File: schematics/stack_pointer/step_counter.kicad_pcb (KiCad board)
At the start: 2 copper layers, 100 x 91 mm, 17 parts, among them U1 74HC00, U2 74HC193, U3 74HC193, U4 74HC193, U5 74HC193, U6 74HC245, U7 74HC245

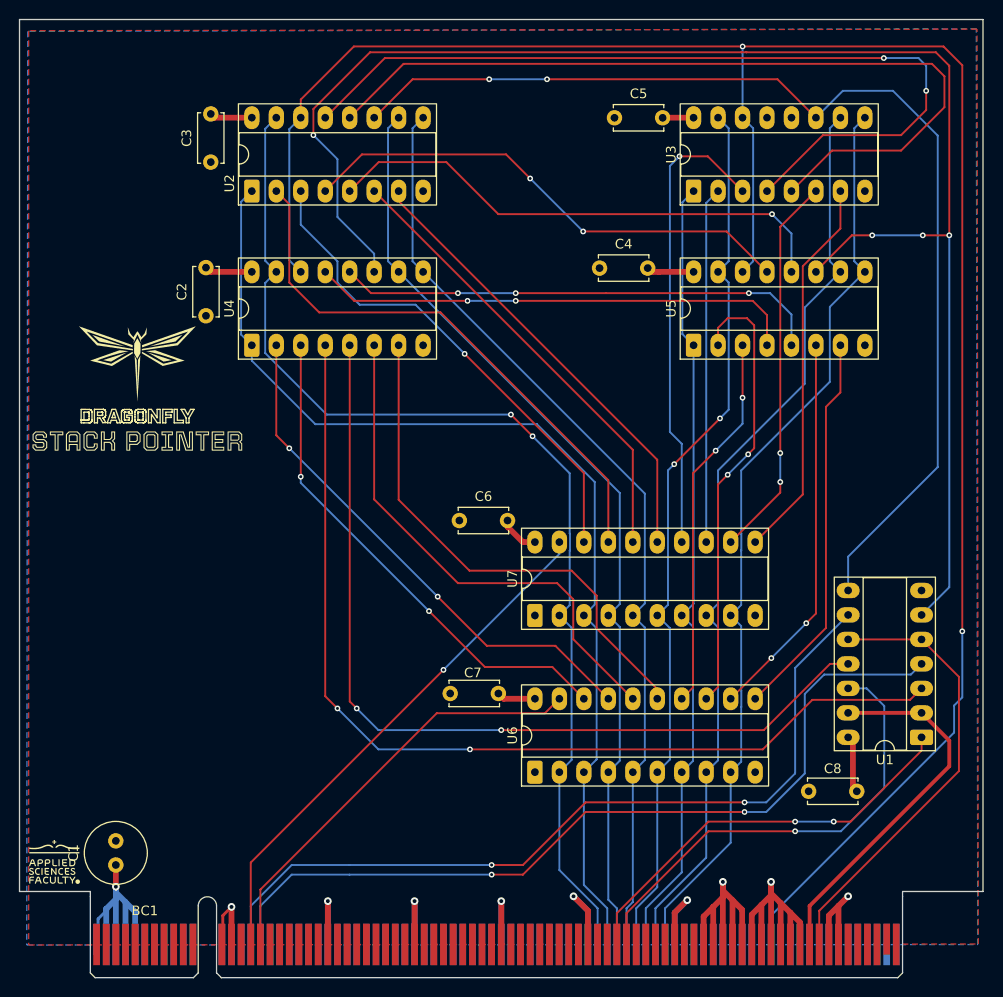
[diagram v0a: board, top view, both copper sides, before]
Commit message: silklayer check
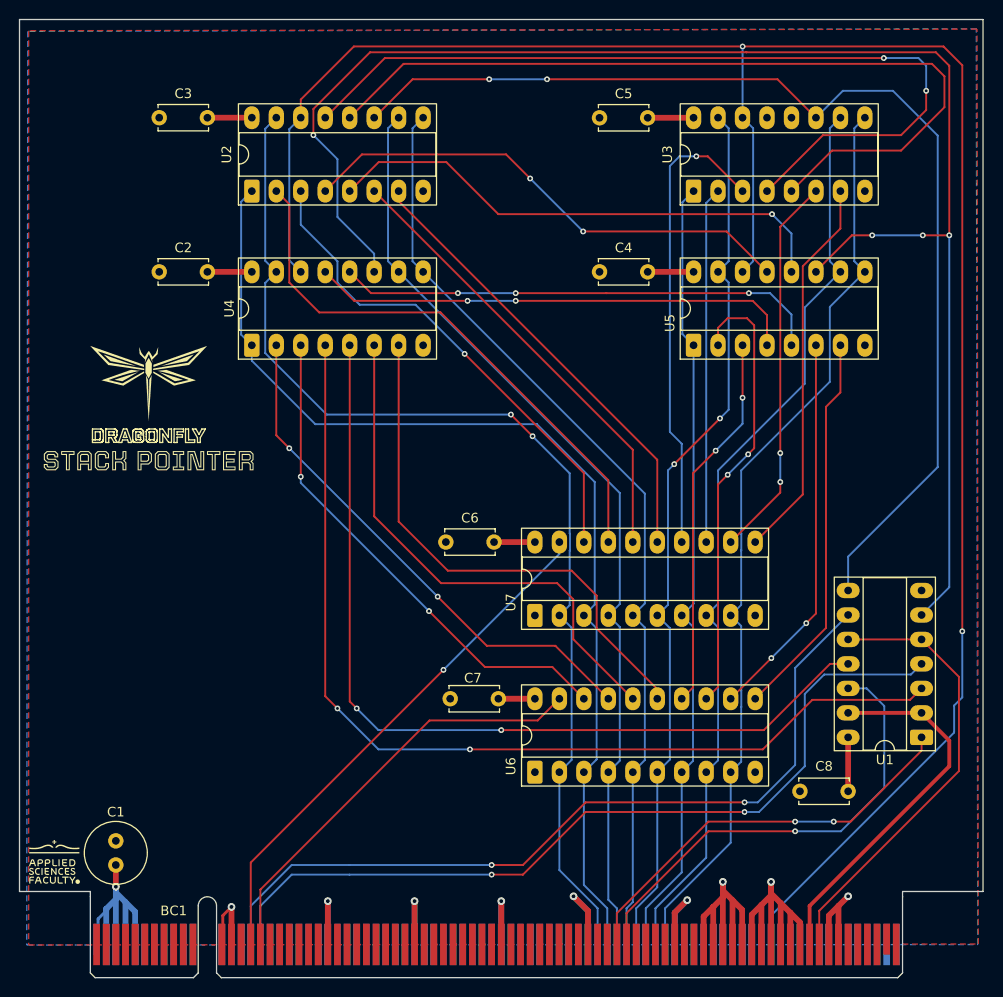
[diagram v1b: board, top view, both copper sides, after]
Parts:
- moved C3 7.06 mm to (121.0, 44.2), turned to 0 degrees
- moved C2 6.66 mm to (121.0, 60.2), turned to 0 degrees
- moved C6 2.64 mm to (150.8, 88.2)
- moved kibuzzard-6911C575 2.35 mm to (119.9, 79.8)
- moved C5 1.55 mm to (166.7, 44.2)
- moved C8 0.90 mm to (192.5, 114.1)
- moved C7 0.55 mm to (156.2, 104.5)
- moved C4 0.39 mm to (166.7, 60.2)
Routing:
- net /DL3: track 54.0 -> 55.3 mm
- net /DL2: track 53.8 -> 54.9 mm
- net VCC: track 59.3 -> 60.0 mm
- net /LSPH: track 84.9 -> 84.4 mm
